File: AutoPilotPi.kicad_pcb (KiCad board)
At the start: 4 copper layers, 29 x 44.7 mm, 105 parts, among them J1 Conn_01x04_MountingPin, J2 Conn_01x04_MountingPin, J3 Conn_01x04_MountingPin, J4 USB_C_Receptacle, SW1 SW_Push, U1 MKDV4GCL-AB, U2 V3S-ALLWINNER, U3 EA3036, U4 GW1N_LV4QN32C6/I5, U5 HMC5883L-TR, U6 SPL06-001, U7 v3s_flight_controller, U8 TLV71312PDBV, Y1 Crystal, Y2 Crystal_GND24_Small

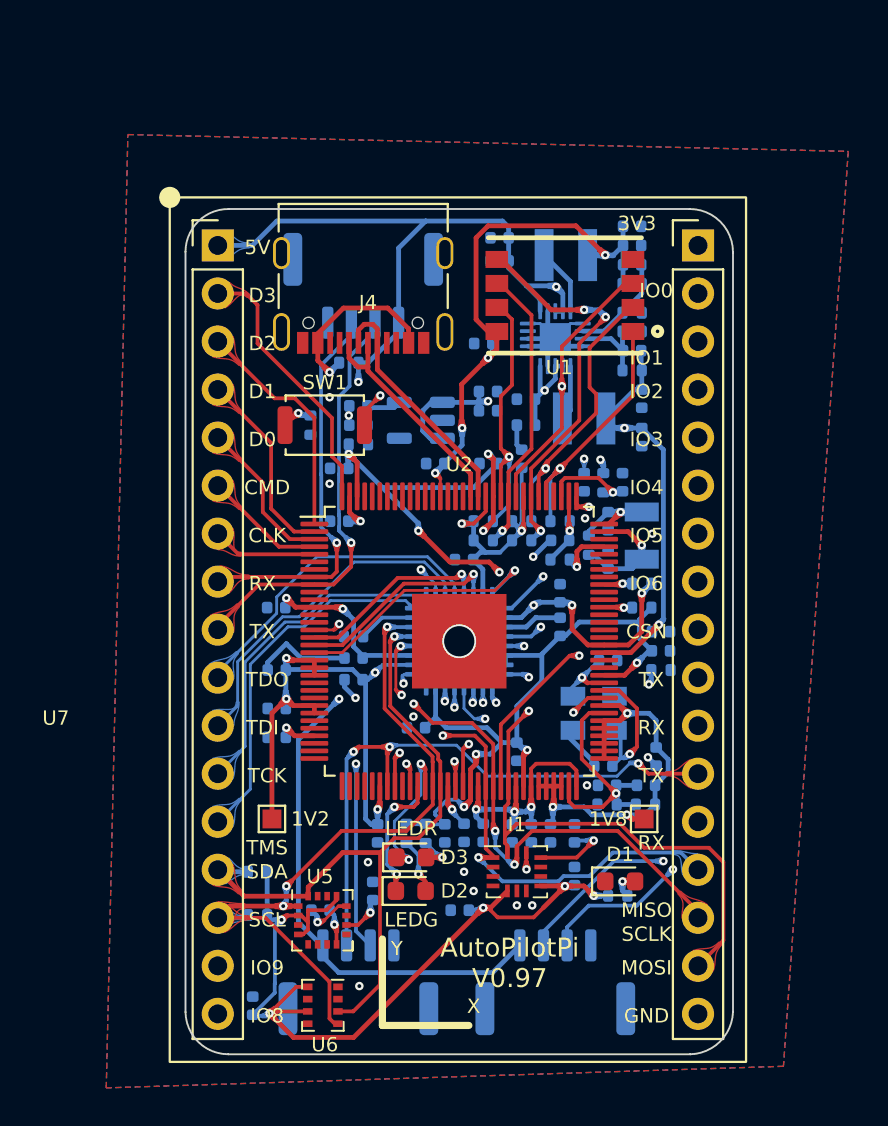
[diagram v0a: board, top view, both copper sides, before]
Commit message: update 2.0
Signed-off-by: huangzzk <huangcmzzk@gmail.com>
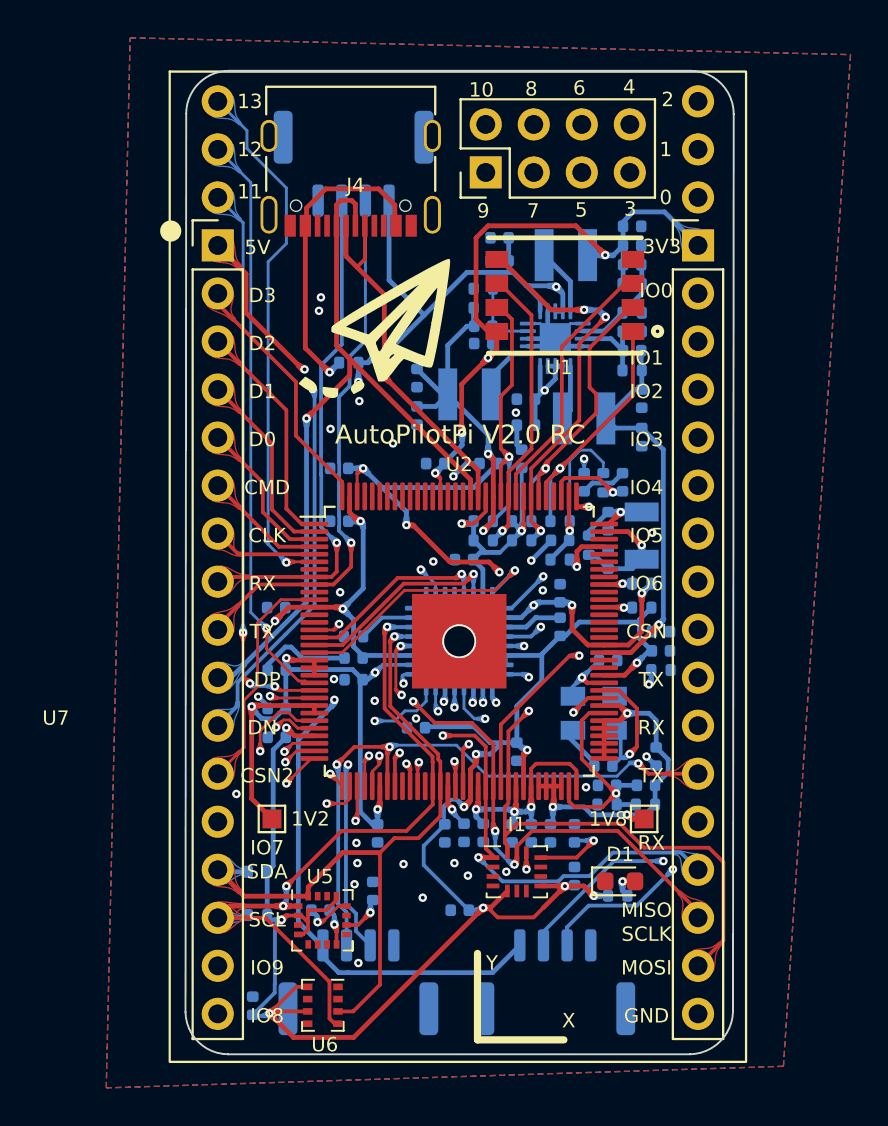
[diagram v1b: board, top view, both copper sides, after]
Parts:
- removed C56: 0.1u, Capacitor_SMD:C_0402_1005Metric
- removed D2, D3: LED, LED_SMD:LED_0603_1608Metric
- removed R25, R26: 10K, Resistor_SMD:R_0402_1005Metric
- removed R27: 499R, Resistor_SMD:R_0402_1005Metric
- removed SW1: SW_Push, Button_Switch_SMD:SW_Push_SPST_NO_Alps_SKRK
- removed U8: TLV71312PDBV, Package_TO_SOT_SMD:SOT-23-5
- added L1: 2.2uH, Inductor_SMD:L_Abracon_ASPI-3012S, B.Cu at (93.0, 56.0)
- added R17: 100K, Resistor_SMD:R_0402_1005Metric, B.Cu at (93.7, 51.5)
- C31: value 4.7uF -> 4.7u
- C34: value 4.7uF -> 0.1u
- C38: value 0.1u -> 220p
- R14: value 0R -> 100k
- R21: value 10K -> NC
- moved R14 10.6 mm to (93.7, 50.4), turned to 0 degrees
- moved C38 7.84 mm to (93.7, 52.4), turned to 0 degrees
- moved J2 6.48 mm to (86.9, 43.8)
- moved J4 6.23 mm to (86.7, 44.6)
- moved C31 3.83 mm to (90.2, 55.2), turned to -90 degrees
- moved C34 3.14 mm to (90.2, 57.1), turned to -90 degrees
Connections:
- net /CSN renamed /USER_CSN1
- C31 pad 1: +1V8 -> +1V2
- C34 pad 1: Net-(C34-Pad1) -> +1V2
- C38 pad 1: Net-(C34-Pad1) -> +1V2
- C38 pad 2: GND -> Net-(C38-Pad2)
- R14 pad 1: Net-(C34-Pad1) -> GND
- R14 pad 2: +1V2 -> Net-(C38-Pad2)
- U2 pad 11: unconnected-(U2-Pad11) -> /USER_CSN2
- U2 pad 13: unconnected-(U2-Pad13) -> /V3s_core/LEDG
- U2 pad 14: unconnected-(U2-Pad14) -> /V3s_core/LEDR
- U2 pad 22: unconnected-(U2-Pad22) -> /GPIO_EXT12
- U2 pad 23: unconnected-(U2-Pad23) -> /GPIO_EXT11
- U2 pad 24: unconnected-(U2-Pad24) -> /GPIO_EXT10
- U2 pad 27: unconnected-(U2-Pad27) -> /GPIO_EXT9
- U2 pad 28: unconnected-(U2-Pad28) -> /GPIO_EXT8
- U2 pad 30: unconnected-(U2-Pad30) -> /GPIO_EXT7
- U2 pad 31: unconnected-(U2-Pad31) -> /GPIO_EXT6
- U2 pad 32: unconnected-(U2-Pad32) -> /GPIO_EXT5
- U2 pad 33: unconnected-(U2-Pad33) -> /GPIO_EXT4
- U2 pad 34: unconnected-(U2-Pad34) -> /GPIO_EXT3
- U2 pad 35: unconnected-(U2-Pad35) -> /GPIO_EXT2
- U2 pad 36: unconnected-(U2-Pad36) -> /GPIO_EXT1
- U2 pad 37: unconnected-(U2-Pad37) -> /GPIO_EXT0
- U2 pad 43: /V3s_core/LEDG -> /FPGA/PLL_IN
- U2 pad 44: /V3s_core/LEDR -> unconnected-(U2-Pad44)
- U2 pad 6: unconnected-(U2-Pad6) -> /GPIO_EXT13
- U3 pad 11: unconnected-(U3-Pad11) -> Net-(L1-Pad2)
- U3 pad 14: unconnected-(U3-Pad14) -> Net-(C38-Pad2)
- U3 pad 9: GND -> +5V
- U4 pad 14: /FPGAIO9 -> /FPGA/PLL_IN
- U4 pad 15: +3V3 -> /FPGAIO9
- U7 pad 10: /FPGA/TDO -> /USB_DP
- U7 pad 11: /FPGA/TDI -> /USB_DN
- U7 pad 12: /FPGA/TCK -> /USER_CSN2
- U7 pad 13: /FPGA/TMS -> /FPGAIO7
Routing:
- net /GPIO_EXT2: track 0.00 -> 48.2 mm, vias 0 -> 1
- net /GPIO_EXT6: track 0.00 -> 42.7 mm, vias 0 -> 1
- net /GPIO_EXT3: track 0.00 -> 42.1 mm, vias 0 -> 1
- net /GPIO_EXT9: track 0.00 -> 42.0 mm, vias 0 -> 1
- net /GPIO_EXT4: track 0.00 -> 41.9 mm, vias 0 -> 1
- net /GPIO_EXT5: track 0.00 -> 41.8 mm, vias 0 -> 1
- net /GPIO_EXT1: track 0.00 -> 41.1 mm, vias 0 -> 1
- net +3V3: track 159.9 -> 200.6 mm, vias 21 -> 20
- net /GPIO_EXT8: track 0.00 -> 40.1 mm, vias 0 -> 1
- net /GPIO_EXT10: track 0.00 -> 38.7 mm, vias 0 -> 1
- net /GPIO_EXT0: track 0.00 -> 38.7 mm, vias 0 -> 1
- net /GPIO_EXT7: track 0.00 -> 37.9 mm, vias 0 -> 1
- net /USB_DN: track 13.0 -> 43.9 mm, vias 0 -> 2
- net /GPIO_EXT12: track 0.00 -> 30.8 mm, vias 0 -> 1
- net /GPIO_EXT11: track 0.00 -> 30.0 mm, vias 0 -> 3
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- added copper zone on In1.Cu, net GND
- removed copper zone on In1.Cu, net +3V3
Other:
- board size 29 x 44.7 mm -> 29 x 52 mm
- board text added: "0"
- board text added: "1"
- board text added: "10"
- board text added: "11"
- board text added: "12"
- board text added: "13"
- board text added: "2"
- board text added: "3"
- board text added: "4"
- board text added: "5"
- board text added: "6"
- board text added: "7"
- board text added: "8"
- board text added: "9"
- board text added: "AutoPilotPi V2.0 RC"
- board text added: "CSN2"
- board text added: "DN"
- board text added: "DP"
- board text added: "IO7"
- board text removed: "AutoPilotPi V0.97"
- board text removed: "LEDG"
- board text removed: "LEDR"
- board text removed: "TCK"
- board text removed: "TDI"
- board text removed: "TDO"
- board text removed: "TMS"
